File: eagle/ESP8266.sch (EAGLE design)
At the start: 7 parts, among them IC1 LM2574HVM-3.3, U1 SN74AHCT125D

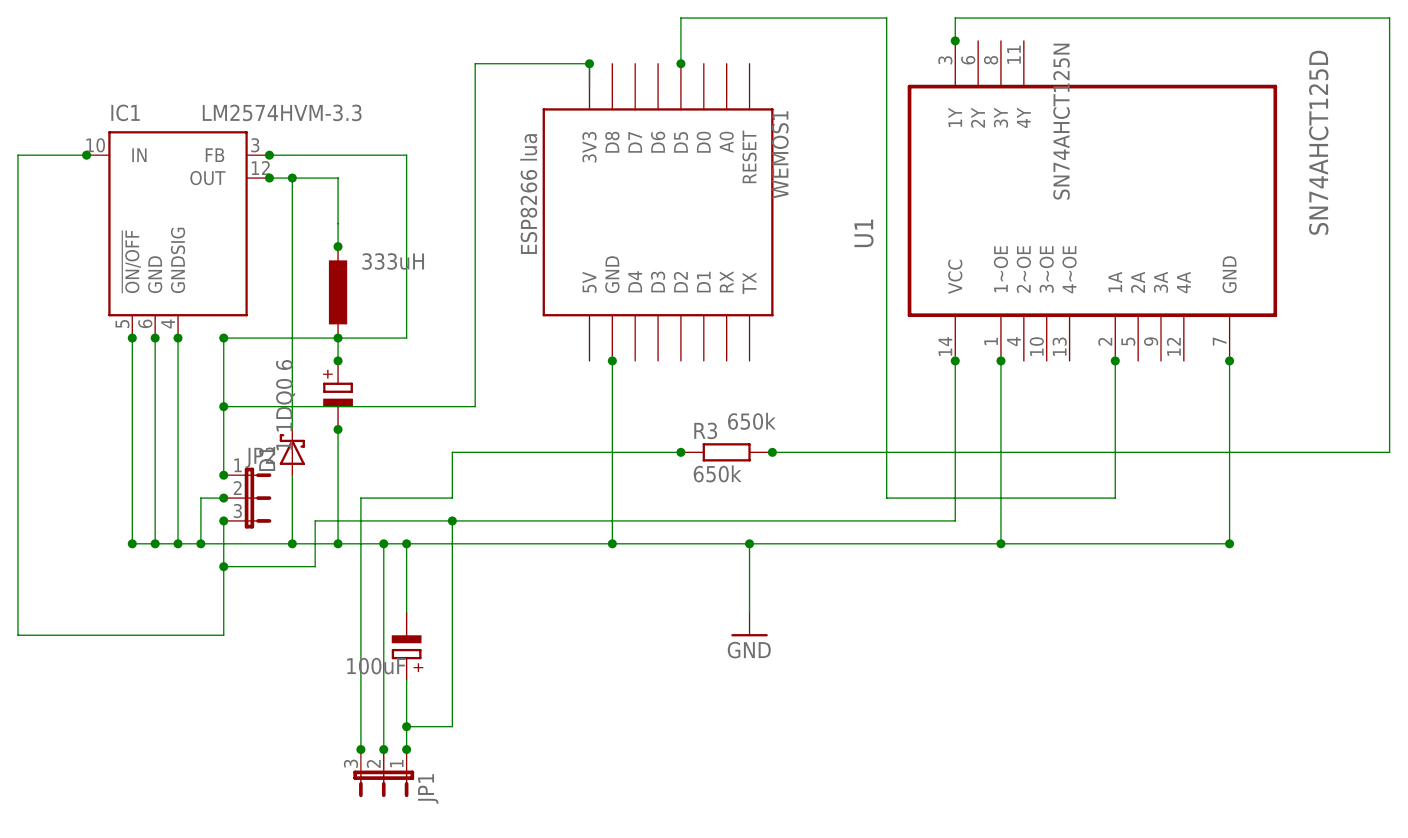
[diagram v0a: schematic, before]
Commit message: schema updated too
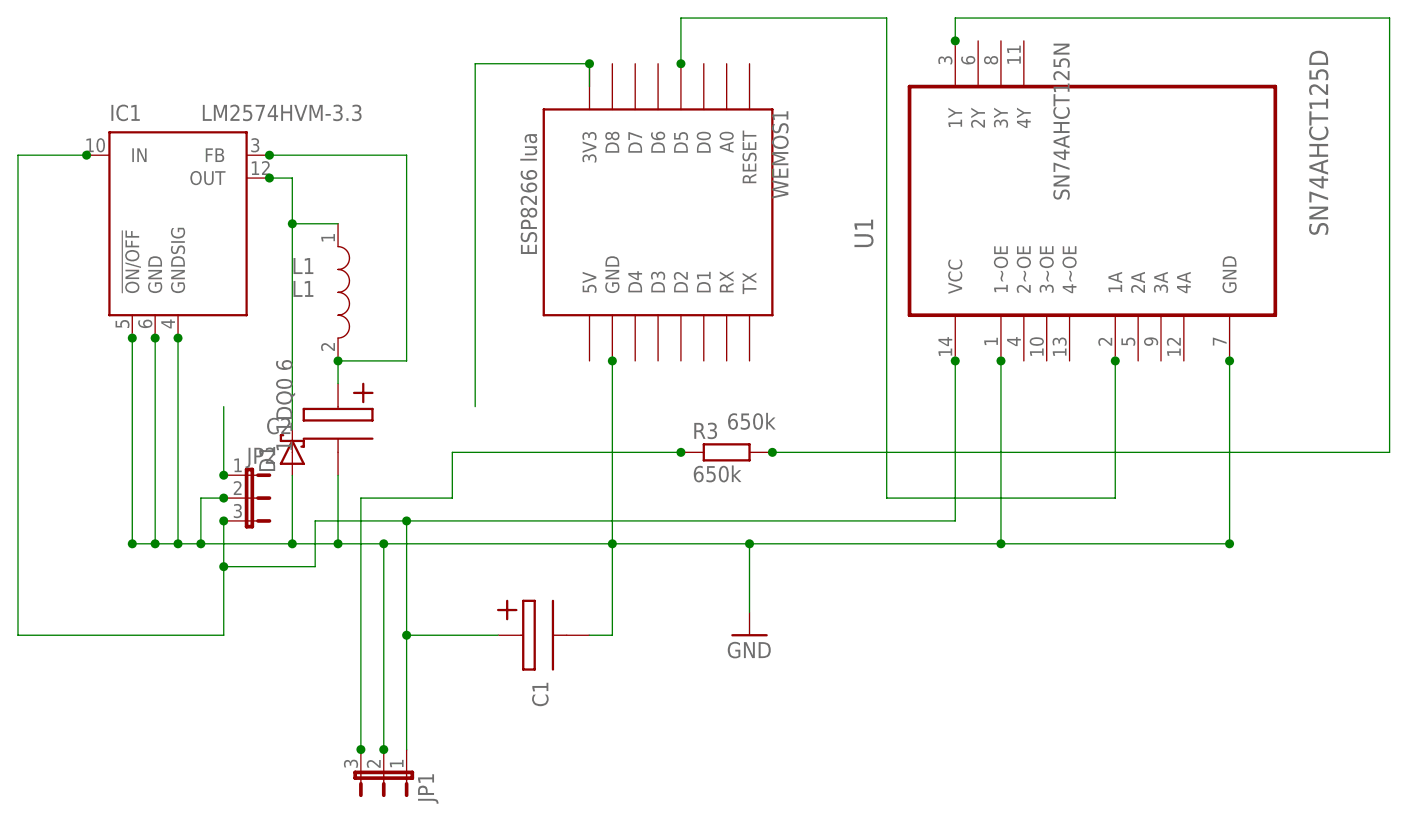
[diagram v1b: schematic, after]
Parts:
- added C1, C2: (no value), e-kondensatoren:GEPOLTER_ELEKTROLYTKONDENSATOR
- added L1: L1, e-spulen-transformatoren:SPULE_ALTERNATIV
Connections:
- removed net N$3: D1.C, IC1.OUT
- new net FB: C2.+, IC1.FB, L1.2
- new net N$4: JP2.1
- new net OUT: D1.C, IC1.OUT, L1.1
- net 5V: now also C1.+
- net GND: now also C1.-, C2.-
- net N$1: no longer IC1.FB, JP2.1
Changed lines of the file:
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@@
 <part name="IC1" library="linear" deviceset="LM2574?-*" device="HVM" technology="3.3"/>
 <part name="JP2" library="jumper" deviceset="JP2E" device=""/>
-<part name="C1" library="docu-dummy" deviceset="ELKO" device="">
-<attribute name="CAPACITY" value="100uF"/>
-</part>
-<part name="C2" library="docu-dummy" deviceset="ELKO" device="">
-<attribute name="CAPACITY" value="220uF"/>
-</part>
 <part name="D1" library="diode" deviceset="SCHOTTKY-DIODE" device="TO92H">
 <attribute name="D" value="1 1DQ0 6"/>
-</part>
-<part name="L1" library="docu-dummy" deviceset="L" device="">
-<attribute name="L1" value="333uH"/>
 </part>
 <part name="R3" library="eagle-ltspice" deviceset="R" device="R0201" value="650k">
@@
 </part>
 <part name="GND1" library="supply1" deviceset="GND" device=""/>
+<part name="C2" library="e-kondensatoren" deviceset="GEPOLTER_ELEKTROLYTKONDENSATOR" device=""/>
+<part name="C1" library="e-kondensatoren" deviceset="GEPOLTER_ELEKTROLYTKONDENSATOR" device=""/>
+<part name="L1" library="e-spulen-transformatoren" deviceset="SPULE_ALTERNATIV" device="" value="L1"/>
 </parts>
 <sheets>
@@
 <instance part="IC1" gate="G$1" x="10.16" y="78.74"/>
 <instance part="JP2" gate="1" x="17.78" y="48.26" rot="R270"/>
-<instance part="C1" gate="G$1" x="35.56" y="30.48" rot="R180">
-<attribute name="CAPACITY" x="35.56" y="30.48" size="1.778" layer="96" rot="R180"/>
-</instance>
-<instance part="C2" gate="G$1" x="27.94" y="60.96">
-<attribute name="CAPACITY" x="27.94" y="60.96" size="1.778" layer="96" display="off"/>
-</instance>
 <instance part="D1" gate="G$1" x="22.86" y="53.34" rot="R90">
 <attribute name="D" x="22.86" y="53.34" size="1.778" layer="96" rot="R90"/>
-</instance>
-<instance part="L1" gate="G$1" x="27.94" y="71.12">
-<attribute name="L1" x="30.48" y="73.66" size="1.778" layer="96"/>
 </instance>
 <instance part="R3" gate="G$1" x="71.12" y="53.34">
@@
 </instance>
 <instance part="GND1" gate="1" x="73.66" y="33.02"/>
+<instance part="C2" gate="G$1" x="27.94" y="55.88"/>
+<instance part="C1" gate="G$1" x="50.8" y="33.02" rot="R90"/>
+<instance part="L1" gate="1" x="27.94" y="71.12"/>
 </instances>
 <busses>
 </busses>
 <nets>
-<net name="N$3" class="0">
+<net name="OUT" class="0">
 <segment>
 <pinref part="IC1" gate="G$1" pin="OUT"/>
 <pinref part="D1" gate="G$1" pin="C"/>
 <wire x1="20.32" y1="83.82" x2="22.86" y2="83.82" width="0.1524" layer="91"/>
-<wire x1="22.86" y1="83.82" x2="22.86" y2="55.88" width="0.1524" layer="91"/>
-<wire x1="22.86" y1="83.82" x2="27.94" y2="83.82" width="0.1524" layer="91"/>
+<wire x1="22.86" y1="83.82" x2="22.86" y2="78.74" width="0.1524" layer="91"/>
 <junction x="20.32" y="83.82"/>
-<junction x="22.86" y="83.82"/>
-<wire x1="27.94" y1="83.82" x2="27.94" y2="78.74" width="0.1524" layer="91"/>
-<wire x1="27.94" y1="76.2" x2="27.94" y2="78.74" width="0.1524" layer="91"/>
-<junction x="27.94" y="76.2"/>
+<pinref part="L1" gate="1" pin="1"/>
+<wire x1="22.86" y1="78.74" x2="22.86" y2="55.88" width="0.1524" layer="91"/>
+<wire x1="27.94" y1="78.74" x2="22.86" y2="78.74" width="0.1524" layer="91"/>
+<junction x="22.86" y="78.74"/>
 </segment>
 </net>
 <net name="5V" class="0">
 <segment>
-<pinref part="JP1" gate="1" pin="1"/>
-<wire x1="35.56" y1="27.94" x2="35.56" y2="22.86" width="0.1524" layer="91"/>
-<wire x1="35.56" y1="22.86" x2="35.56" y2="20.32" width="0.1524" layer="91"/>
-<wire x1="35.56" y1="22.86" x2="40.64" y2="22.86" width="0.1524" layer="91"/>
-<wire x1="40.64" y1="22.86" x2="40.64" y2="45.72" width="0.1524" layer="91"/>
-<junction x="35.56" y="22.86"/>
-<junction x="35.56" y="20.32"/>
-<wire x1="40.64" y1="45.72" x2="96.52" y2="45.72" width="0.1524" layer="91"/>
+<wire x1="25.4" y1="45.72" x2="35.56" y2="45.72" width="0.1524" layer="91"/>
+<wire x1="35.56" y1="45.72" x2="96.52" y2="45.72" width="0.1524" layer="91"/>
 <wire x1="96.52" y1="45.72" x2="96.52" y2="63.5" width="0.1524" layer="91"/>
 <pinref part="U1" gate="A" pin="VCC"/>
 <junction x="96.52" y="63.5"/>
-<wire x1="40.64" y1="45.72" x2="25.4" y2="45.72" width="0.1524" layer="91"/>
 <wire x1="25.4" y1="45.72" x2="25.4" y2="40.64" width="0.1524" layer="91"/>
 <pinref part="JP2" gate="1" pin="3"/>
@@
 <wire x1="25.4" y1="40.64" x2="15.24" y2="40.64" width="0.1524" layer="91"/>
 <junction x="15.24" y="40.64"/>
-<junction x="40.64" y="45.72"/>
+<pinref part="JP1" gate="1" pin="1"/>
+<wire x1="35.56" y1="20.32" x2="35.56" y2="33.02" width="0.1524" layer="91"/>
+<junction x="35.56" y="45.72"/>
+<pinref part="C1" gate="G$1" pin="+"/>
+<wire x1="35.56" y1="33.02" x2="35.56" y2="45.72" width="0.1524" layer="91"/>
+<wire x1="45.72" y1="33.02" x2="35.56" y2="33.02" width="0.1524" layer="91"/>
+<junction x="35.56" y="33.02"/>
 </segment>
 </net>
@@
 <net name="SIGOUT(5V)" class="0">
 <segment>
-<pinref part="JP1" gate="1" pin="3"/>
 <wire x1="40.64" y1="53.34" x2="40.64" y2="48.26" width="0.1524" layer="91"/>
-<wire x1="40.64" y1="48.26" x2="30.48" y2="48.26" width="0.1524" layer="91"/>
-<wire x1="30.48" y1="48.26" x2="30.48" y2="20.32" width="0.1524" layer="91"/>
 <pinref part="R3" gate="G$1" pin="1"/>
 <wire x1="66.04" y1="53.34" x2="40.64" y2="53.34" width="0.1524" layer="91"/>
+<junction x="66.04" y="53.34"/>
+<pinref part="JP1" gate="1" pin="3"/>
+<wire x1="30.48" y1="48.26" x2="30.48" y2="20.32" width="0.1524" layer="91"/>
 <junction x="30.48" y="20.32"/>
-<junction x="66.04" y="53.34"/>
+<wire x1="30.48" y1="48.26" x2="40.64" y2="48.26" width="0.1524" layer="91"/>
 </segment>
 </net>
@@
 <wire x1="101.6" y1="43.18" x2="73.66" y2="43.18" width="0.1524" layer="91"/>
 <wire x1="73.66" y1="43.18" x2="58.42" y2="43.18" width="0.1524" layer="91"/>
-<wire x1="58.42" y1="43.18" x2="35.56" y2="43.18" width="0.1524" layer="91"/>
-<wire x1="35.56" y1="43.18" x2="33.02" y2="43.18" width="0.1524" layer="91"/>
+<wire x1="58.42" y1="43.18" x2="33.02" y2="43.18" width="0.1524" layer="91"/>
 <wire x1="33.02" y1="43.18" x2="27.94" y2="43.18" width="0.1524" layer="91"/>
 <wire x1="27.94" y1="43.18" x2="22.86" y2="43.18" width="0.1524" layer="91"/>
@@
 <pinref part="JP1" gate="1" pin="2"/>
 <wire x1="33.02" y1="43.18" x2="33.02" y2="20.32" width="0.1524" layer="91"/>
-<wire x1="35.56" y1="35.56" x2="35.56" y2="43.18" width="0.1524" layer="91"/>
 <pinref part="WEMOS1" gate="D1" pin="GND"/>
 <wire x1="58.42" y1="63.5" x2="58.42" y2="43.18" width="0.1524" layer="91"/>
@@
 <junction x="10.16" y="43.18"/>
 <junction x="15.24" y="48.26"/>
-<junction x="35.56" y="43.18"/>
 <junction x="33.02" y="20.32"/>
 <junction x="58.42" y="63.5"/>
@@
 <junction x="12.7" y="43.18"/>
 <junction x="33.02" y="43.18"/>
-<wire x1="27.94" y1="43.18" x2="27.94" y2="55.88" width="0.1524" layer="91"/>
+<junction x="127" y="63.5"/>
+<pinref part="C2" gate="G$1" pin="-"/>
+<wire x1="27.94" y1="43.18" x2="27.94" y2="50.8" width="0.1524" layer="91"/>
 <junction x="27.94" y="43.18"/>
-<junction x="27.94" y="55.88"/>
-<junction x="127" y="63.5"/>
+<pinref part="C1" gate="G$1" pin="-"/>
+<wire x1="55.88" y1="33.02" x2="58.42" y2="33.02" width="0.1524" layer="91"/>
+<wire x1="58.42" y1="33.02" x2="58.42" y2="43.18" width="0.1524" layer="91"/>
 </segment>
 </net>
 <net name="N$1" class="0">
+<segment>
+<pinref part="WEMOS1" gate="D1" pin="3V3"/>
+<wire x1="55.88" y1="96.52" x2="55.88" y2="93.98" width="0.1524" layer="91"/>
+<wire x1="43.18" y1="58.42" x2="43.18" y2="96.52" width="0.1524" layer="91"/>
+<wire x1="43.18" y1="96.52" x2="55.88" y2="96.52" width="0.1524" layer="91"/>
+<junction x="55.88" y="96.52"/>
+</segment>
+</net>
+<net name="FB" class="0">
 <segment>
 <pinref part="IC1" gate="G$1" pin="FB"/>
 <junction x="20.32" y="86.36"/>
 <wire x1="20.32" y1="86.36" x2="35.56" y2="86.36" width="0.1524" layer="91"/>
-<wire x1="35.56" y1="86.36" x2="35.56" y2="66.04" width="0.1524" layer="91"/>
-<pinref part="WEMOS1" gate="D1" pin="3V3"/>
-<wire x1="55.88" y1="96.52" x2="55.88" y2="93.98" width="0.1524" layer="91"/>
+<wire x1="35.56" y1="86.36" x2="35.56" y2="63.5" width="0.1524" layer="91"/>
+<pinref part="C2" gate="G$1" pin="+"/>
+<wire x1="27.94" y1="63.5" x2="27.94" y2="60.96" width="0.1524" layer="91"/>
+<wire x1="35.56" y1="63.5" x2="27.94" y2="63.5" width="0.1524" layer="91"/>
+<pinref part="L1" gate="1" pin="2"/>
+<junction x="27.94" y="63.5"/>
+</segment>
+</net>
+<net name="N$4" class="0">
+<segment>
 <pinref part="JP2" gate="1" pin="1"/>
 <wire x1="15.24" y1="50.8" x2="15.24" y2="58.42" width="0.1524" layer="91"/>
-<wire x1="15.24" y1="58.42" x2="43.18" y2="58.42" width="0.1524" layer="91"/>
-<wire x1="43.18" y1="58.42" x2="43.18" y2="96.52" width="0.1524" layer="91"/>
-<wire x1="43.18" y1="96.52" x2="55.88" y2="96.52" width="0.1524" layer="91"/>
 <junction x="15.24" y="50.8"/>
-<junction x="55.88" y="96.52"/>
-<junction x="15.24" y="58.42"/>
-<wire x1="35.56" y1="66.04" x2="27.94" y2="66.04" width="0.1524" layer="91"/>
-<wire x1="27.94" y1="66.04" x2="15.24" y2="66.04" width="0.1524" layer="91"/>
-<wire x1="15.24" y1="66.04" x2="15.24" y2="58.42" width="0.1524" layer="91"/>
-<wire x1="27.94" y1="66.04" x2="27.94" y2="63.5" width="0.1524" layer="91"/>
-<junction x="27.94" y="66.04"/>
-<junction x="15.24" y="66.04"/>
-<junction x="27.94" y="63.5"/>
-</segment>
-</net>
+</segment>
+</net>
